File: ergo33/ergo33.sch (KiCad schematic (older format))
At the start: 113 parts, among them SW1 SW_Push, SW46 Rotary_Encoder_Switch, U1 ATmega32U4-AU, Y1 16MHz

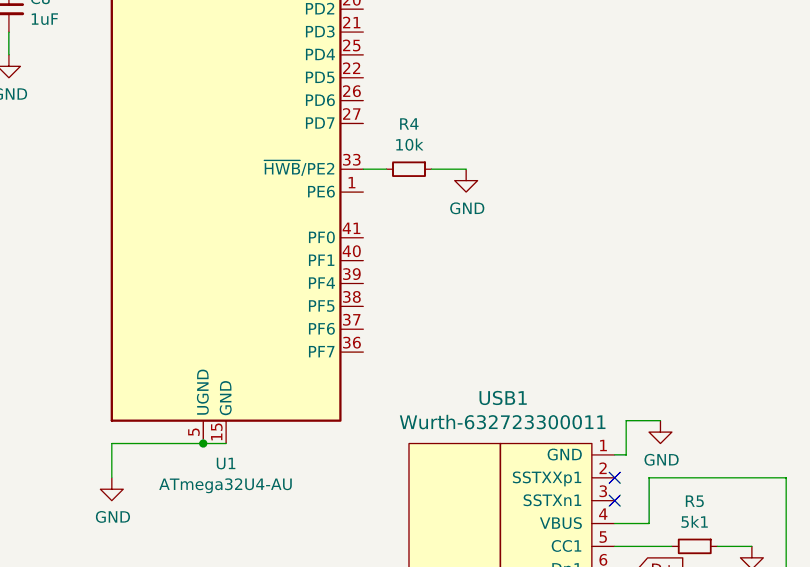
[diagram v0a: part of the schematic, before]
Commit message: Rerouting ergo33
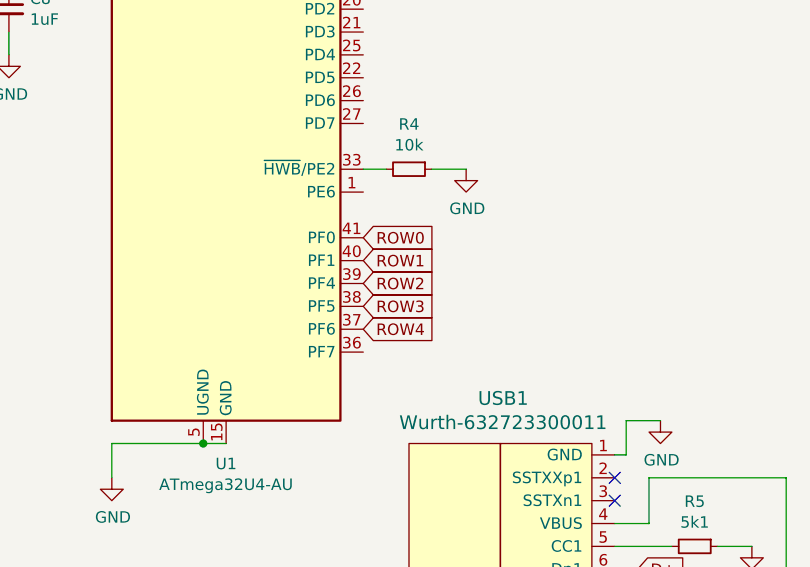
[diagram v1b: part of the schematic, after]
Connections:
- net ROW0: now also U1.41 (PF0)
- net ROW1: now also U1.40 (PF1)
- net ROW2: now also U1.39 (PF4)
- net ROW3: now also U1.38 (PF5)
- net ROW4: now also U1.37 (PF6)
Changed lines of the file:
@@
 Text GLabel 4850 5850 3    50   Input ~ 0
 PWR_IN
+Text GLabel 3150 4100 2    50   Input ~ 0
+ROW0
+Text GLabel 3150 4200 2    50   Input ~ 0
+ROW1
+Text GLabel 3150 4300 2    50   Input ~ 0
+ROW2
+Text GLabel 3150 4400 2    50   Input ~ 0
+ROW3
+Text GLabel 3150 4500 2    50   Input ~ 0
+ROW4
 $EndSCHEMATC

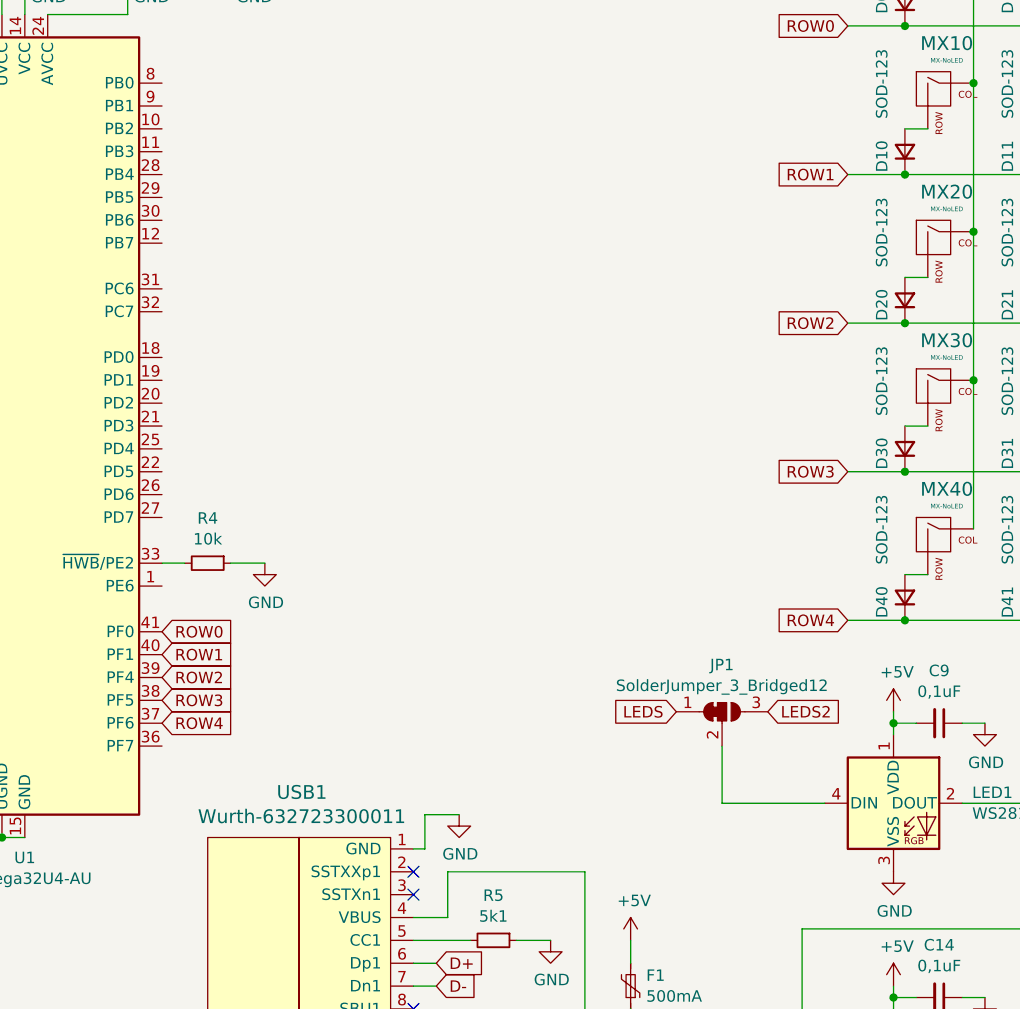
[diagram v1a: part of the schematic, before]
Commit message: Finish ergo33 routing v1
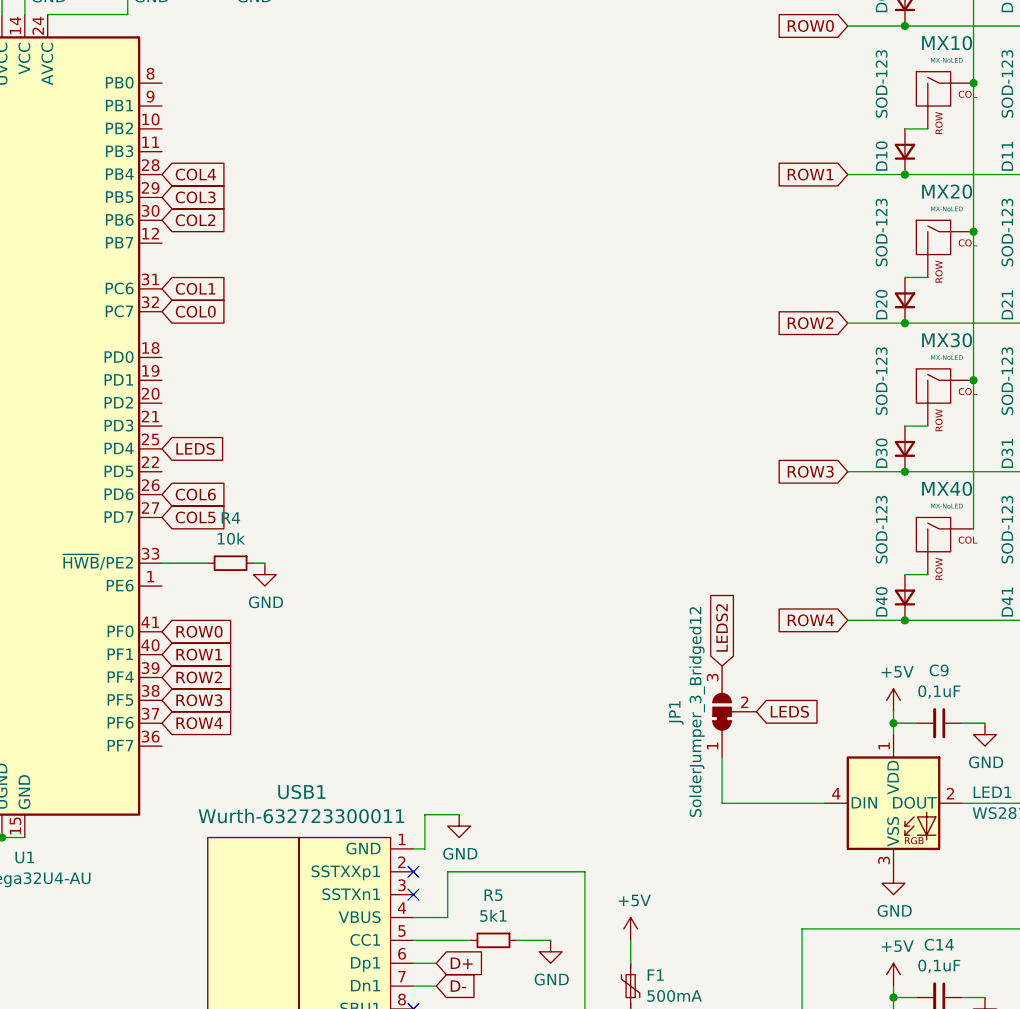
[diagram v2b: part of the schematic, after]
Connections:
- net COL0: now also U1.32 (PC7)
- net COL1: now also U1.31 (PC6)
- net COL2: now also U1.30 (PB6)
- net COL3: now also U1.29 (PB5)
- net COL4: now also U1.28 (PB4)
- net COL5: now also U1.27 (PD7)
- net COL6: now also U1.26 (PD6)
- net LEDS: now also JP1.2 (C), U1.25 (PD4); no longer JP1.1 (A)
- net at LED1.4 (DIN): now also JP1.1 (A); no longer JP1.2 (C)
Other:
- moved on the sheet: JP1, R4
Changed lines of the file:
@@
 L Device:R_Small R4
 U 1 1 5F14E7F9
-P 3350 3800
-F 0 "R4" V 3154 3800 50  0000 C CNN
-F 1 "10k" V 3245 3800 50  0000 C CNN
-F 2 "Resistor_SMD:R_0805_2012Metric" H 3350 3800 50  0001 C CNN
-F 3 "~" H 3350 3800 50  0001 C CNN
-	1    3350 3800
+P 3450 3800
+F 0 "R4" V 3254 3800 50  0000 C CNN
+F 1 "10k" V 3345 3800 50  0000 C CNN
+F 2 "Resistor_SMD:R_0805_2012Metric" H 3450 3800 50  0001 C CNN
+F 3 "~" H 3450 3800 50  0001 C CNN
+	1    3450 3800
 	0    1    1    0
 $EndComp
@@
 	1    0    0    -1
 $EndComp
-Wire Wire Line
-	3150 3800 3250 3800
-Wire Wire Line
-	3450 3800 3600 3800
 $Comp
 L Device:R_Small R3
@@
 	1    0    0    -1
 $EndComp
-Text GLabel 5400 4450 0    50   Input ~ 0
+Text GLabel 5750 4450 2    50   Input ~ 0
 LEDS
 Wire Wire Line
@@
 	1300 2000 1200 2000
 Wire Wire Line
-	5600 4600 5600 4850
-Wire Wire Line
 	10800 6050 10800 5700
 Connection ~ 10800 6050
 Wire Wire Line
 	10800 6050 10950 6050
-Text GLabel 5800 4450 2    50   Input ~ 0
+Text GLabel 5600 4250 1    50   Input ~ 0
 LEDS2
 Wire Wire Line
@@
 F 3 "~" H 5600 4450 50  0001 C CNN
 	1    5600 4450
-	1    0    0    -1
+	0    -1   -1   0
 $EndComp
 Wire Wire Line
@@
 Text GLabel 3150 4500 2    50   Input ~ 0
 ROW4
+Wire Wire Line
+	5600 4650 5600 4850
+Text GLabel 3150 2700 2    50   Input ~ 0
+COL0
+Text GLabel 3150 2600 2    50   Input ~ 0
+COL1
+Text GLabel 3150 2300 2    50   Input ~ 0
+COL2
+Text GLabel 3150 2200 2    50   Input ~ 0
+COL3
+Text GLabel 3150 2100 2    50   Input ~ 0
+COL4
+Text GLabel 3150 3600 2    50   Input ~ 0
+COL5
+Wire Wire Line
+	3550 3800 3600 3800
+Wire Wire Line
+	3150 3800 3350 3800
+Text GLabel 3150 3500 2    50   Input ~ 0
+COL6
+Text GLabel 3150 3300 2    50   Input ~ 0
+LEDS
 $EndSCHEMATC
